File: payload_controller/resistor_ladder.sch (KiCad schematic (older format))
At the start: 35 parts, among them U1 74HC590, U10 ADG841YKSZ-500RL7, U10 OPA2387, U11 ADG841YKSZ-500RL7, U11 MCP4725xxx-xCH, U12 ADG841YKSZ-500RL7, U13 ADG841YKSZ-500RL7, U6 ADG841YKSZ-500RL7, U7 ADG841YKSZ-500RL7, U8 ADG841YKSZ-500RL7, U9 ADG841YKSZ-500RL7

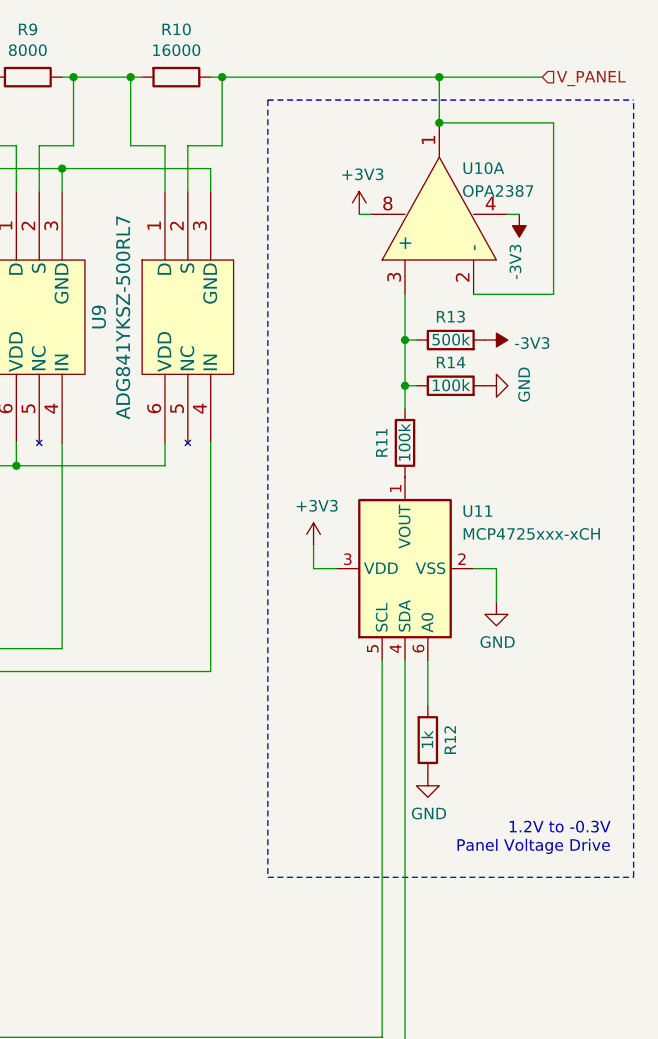
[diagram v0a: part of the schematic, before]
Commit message: Continuing layout
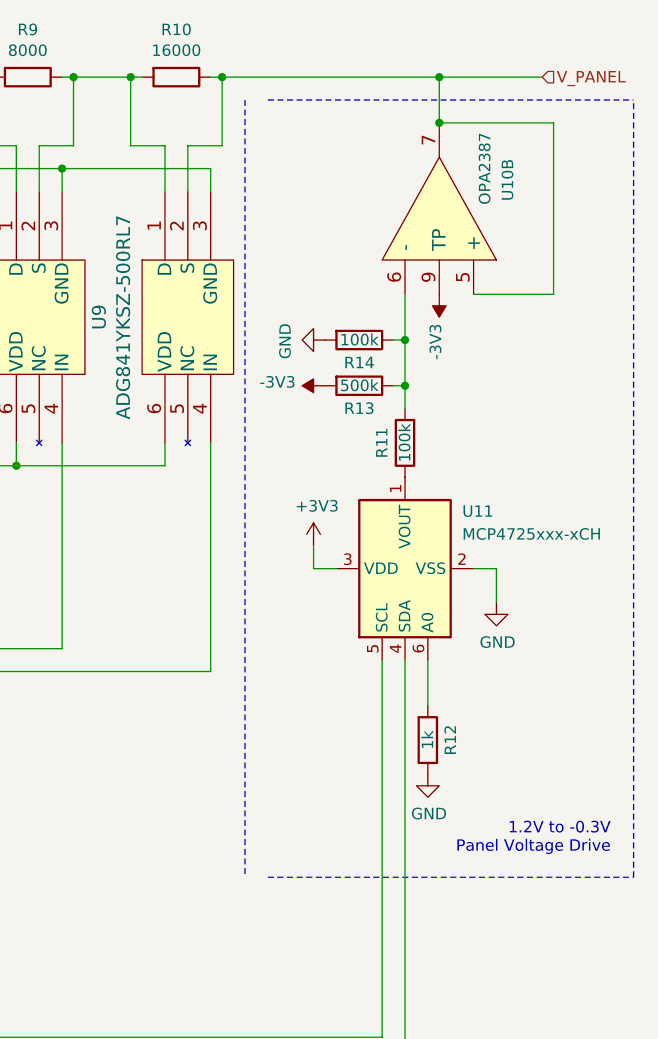
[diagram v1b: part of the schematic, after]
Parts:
- removed U10: OPA2387, Package_SON:WSON-8-1EP_2x2mm_P0.5mm_EP0.9x1.6mm, symbol OPA2387:OPA2387
- added unit 2 of U10
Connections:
- net -3V3: now also U10.9 (TP)
- net V_PANEL: now also U10.5 (+), U10.7
- net at R11.2, R13.1, R14.1: now also U10.6 (-)
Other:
- moved on the sheet: R13, R14
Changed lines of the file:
@@
 	-1   0    0    1
-$EndComp
-$Comp
-L Device:R R14
-U 1 1 6395E4CC
-P 9550 2700
-F 0 "R14" V 9650 2700 50  0000 C CNN
-F 1 "100k" V 9550 2700 50  0000 C CNN
-F 2 "Resistor_SMD:R_0603_1608Metric" V 9480 2700 50  0001 C CNN
-F 3 "~" H 9550 2700 50  0001 C CNN
-	1    9550 2700
-	0    -1   -1   0
-$EndComp
-$Comp
-L power:GND #PWR0134
-U 1 1 6395EDA9
-P 9700 2700
-F 0 "#PWR0134" H 9700 2450 50  0001 C CNN
-F 1 "GND" H 9705 2527 50  0000 C CNN
-F 2 "" H 9700 2700 50  0001 C CNN
-F 3 "" H 9700 2700 50  0001 C CNN
-	1    9700 2700
-	0    -1   -1   0
 $EndComp
 Wire Wire Line
@@
 Wire Wire Line
 	9500 1350 9500 1550
-$Comp
-L power:-3V3 #PWR?
-U 1 1 638EAACA
-P 9700 2500
-AR Path="/63C503EE/638EAACA" Ref="#PWR?"  Part="1"
-AR Path="/635FEB2F/638EAACA" Ref="#PWR0136"  Part="1"
-F 0 "#PWR0136" H 9700 2600 50  0001 C CNN
-F 1 "-3V3" V 9715 2628 50  0000 L CNN
-F 2 "" H 9700 2500 50  0001 C CNN
-F 3 "" H 9700 2500 50  0001 C CNN
-	1    9700 2500
-	0    1    1    0
-$EndComp
 Wire Wire Line
 	9650 2300 10000 2300
@@
 Wire Wire Line
 	10000 1550 9500 1550
-$Comp
-L Device:R R13
-U 1 1 6391F434
-P 9550 2500
-F 0 "R13" V 9650 2500 50  0000 C CNN
-F 1 "500k" V 9550 2500 50  0000 C CNN
-F 2 "Resistor_SMD:R_0603_1608Metric" V 9480 2500 50  0001 C CNN
-F 3 "~" H 9550 2500 50  0001 C CNN
-	1    9550 2500
-	0    -1   -1   0
-$EndComp
 Connection ~ 9500 1350
 Wire Wire Line
 	9500 1350 9950 1350
-Wire Wire Line
-	9350 2300 9350 2500
-Wire Wire Line
-	9400 2700 9350 2700
-Wire Wire Line
-	9400 2500 9350 2500
-Connection ~ 9350 2500
-Wire Wire Line
-	9350 2500 9350 2700
-Wire Wire Line
-	9350 2800 9350 2700
-Connection ~ 9350 2700
 Wire Wire Line
 	9450 3900 9450 4100
@@
 	9350 3900 9350 5650
 Wire Notes Line
-	8750 1450 8750 4850
+	8650 1450 8650 4850
 Wire Notes Line
 	8750 4850 10350 4850
@@
 	1700 3750 2050 3750
 $Comp
-L OPA2387:OPA2387 U10
-U 1 1 6382E466
-P 9500 2050
-F 0 "U10" V 9800 1950 50  0000 R CNN
-F 1 "OPA2387" V 9700 1950 50  0000 R CNN
-F 2 "Package_SON:WSON-8-1EP_2x2mm_P0.5mm_EP0.9x1.6mm" H 9900 2250 50  0001 C CNN
-F 3 "" H 9900 2250 50  0001 C CNN
-	1    9500 2050
-	0    -1   -1   0
-$EndComp
-Connection ~ 9500 1550
-$Comp
 L power:-3V3 #PWR?
 U 1 1 6383D96E
-P 9850 1950
+P 9500 2300
 AR Path="/63C503EE/6383D96E" Ref="#PWR?"  Part="1"
 AR Path="/635FEB2F/6383D96E" Ref="#PWR0128"  Part="1"
-F 0 "#PWR0128" H 9850 2050 50  0001 C CNN
-F 1 "-3V3" V 9865 2078 50  0000 L CNN
-F 2 "" H 9850 1950 50  0001 C CNN
-F 3 "" H 9850 1950 50  0001 C CNN
-	1    9850 1950
+F 0 "#PWR0128" H 9500 2400 50  0001 C CNN
+F 1 "-3V3" V 9515 2428 50  0000 L CNN
+F 2 "" H 9500 2300 50  0001 C CNN
+F 3 "" H 9500 2300 50  0001 C CNN
+	1    9500 2300
 	-1   0    0    1
 $EndComp
-$Comp
-L power:+3V3 #PWR0135
-U 1 1 6383DF99
-P 9150 1950
-F 0 "#PWR0135" H 9150 1800 50  0001 C CNN
-F 1 "+3V3" H 9165 2123 50  0000 C CNN
-F 2 "" H 9150 1950 50  0001 C CNN
-F 3 "" H 9150 1950 50  0001 C CNN
-	1    9150 1950
-	1    0    0    -1
-$EndComp
-Wire Wire Line
-	9850 1950 9800 1950
-Wire Wire Line
-	9150 1950 9200 1950
 Connection ~ 3950 1750
 Wire Wire Line
@@
 	0    1    1    0
 $EndComp
+$Comp
+L OPA2387:OPA2387 U?
+U 2 1 63A95D48
+P 9500 2050
+AR Path="/63C503EE/63A95D48" Ref="U?"  Part="2"
+AR Path="/635FEB2F/63A95D48" Ref="U10"  Part="2"
+F 0 "U10" H 9750 2350 50  0000 C CNN
+F 1 "OPA2387" H 9800 2250 50  0000 C CNN
+F 2 "Package_SON:WSON-8-1EP_2x2mm_P0.5mm_EP0.9x1.6mm" H 9900 2250 50  0001 C CNN
+F 3 "" H 9900 2250 50  0001 C CNN
+	2    9500 2050
+	0    1    -1   0
+$EndComp
+Connection ~ 9500 1550
+Connection ~ 9350 2700
+Connection ~ 9350 2500
+Wire Wire Line
+	9350 2300 9350 2500
+Wire Wire Line
+	9350 2800 9350 2700
+Wire Wire Line
+	9350 2500 9350 2700
+Wire Wire Line
+	9300 2700 9350 2700
+Wire Wire Line
+	9300 2500 9350 2500
+$Comp
+L Device:R R13
+U 1 1 6391F434
+P 9150 2700
+F 0 "R13" V 9250 2700 50  0000 C CNN
+F 1 "500k" V 9150 2700 50  0000 C CNN
+F 2 "Resistor_SMD:R_0603_1608Metric" V 9080 2700 50  0001 C CNN
+F 3 "~" H 9150 2700 50  0001 C CNN
+	1    9150 2700
+	0    1    1    0
+$EndComp
+$Comp
+L power:-3V3 #PWR?
+U 1 1 638EAACA
+P 9000 2700
+AR Path="/63C503EE/638EAACA" Ref="#PWR?"  Part="1"
+AR Path="/635FEB2F/638EAACA" Ref="#PWR0136"  Part="1"
+F 0 "#PWR0136" H 9000 2800 50  0001 C CNN
+F 1 "-3V3" V 9015 2828 50  0000 L CNN
+F 2 "" H 9000 2700 50  0001 C CNN
+F 3 "" H 9000 2700 50  0001 C CNN
+	1    9000 2700
+	0    -1   -1   0
+$EndComp
+$Comp
+L power:GND #PWR0134
+U 1 1 6395EDA9
+P 9000 2500
+F 0 "#PWR0134" H 9000 2250 50  0001 C CNN
+F 1 "GND" H 9005 2327 50  0000 C CNN
+F 2 "" H 9000 2500 50  0001 C CNN
+F 3 "" H 9000 2500 50  0001 C CNN
+	1    9000 2500
+	0    1    1    0
+$EndComp
+$Comp
+L Device:R R14
+U 1 1 6395E4CC
+P 9150 2500
+F 0 "R14" V 9250 2500 50  0000 C CNN
+F 1 "100k" V 9150 2500 50  0000 C CNN
+F 2 "Resistor_SMD:R_0603_1608Metric" V 9080 2500 50  0001 C CNN
+F 3 "~" H 9150 2500 50  0001 C CNN
+	1    9150 2500
+	0    1    1    0
+$EndComp
